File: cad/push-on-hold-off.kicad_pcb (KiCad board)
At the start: 2 copper layers, 22.9 x 12.7 mm, 17 parts, among them P1 CONN_01X04, P2 CONN_01X04, Q1 IRF7309IPBF, SW1 SW_PUSH_SMALL

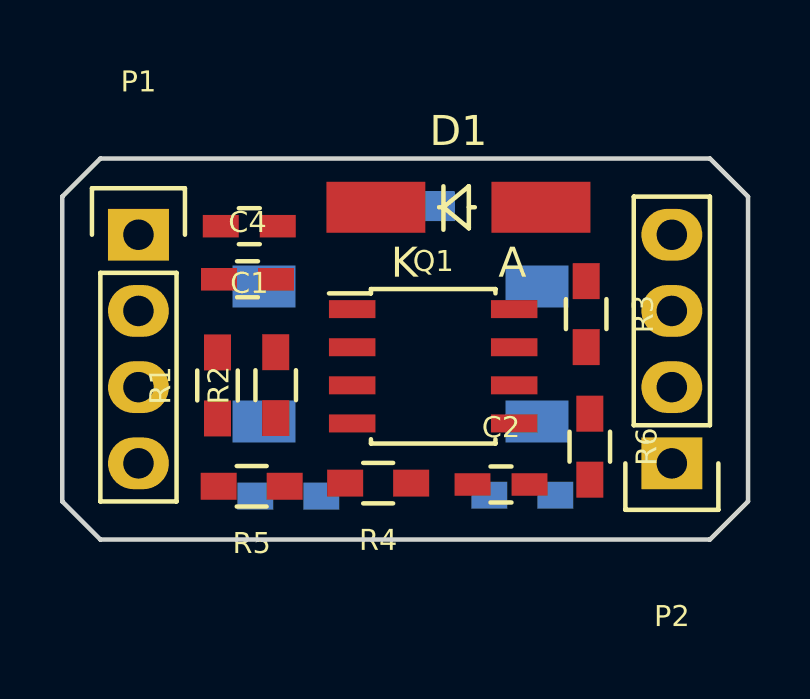
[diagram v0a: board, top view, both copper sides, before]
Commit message: Route the board
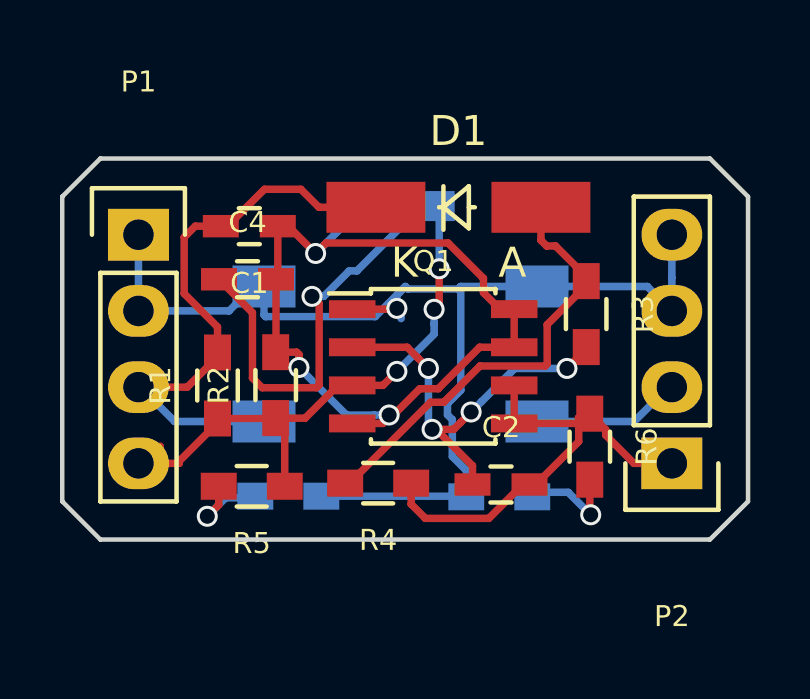
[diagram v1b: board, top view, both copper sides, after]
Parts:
- moved LED2 0.77 mm to (230.5, 111.6), turned to 0 degrees
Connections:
- C4 pad 1: /Vin -> Net-(C4-Pad1)
- JP1 pad 2: /Vin -> Net-(C4-Pad1)
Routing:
- net GND: track 0.00 -> 40.5 mm, vias 0 -> 1
- net Net-(C1-Pad1): track 0.00 -> 28.8 mm, vias 0 -> 3
- net /Button: track 0.00 -> 24.5 mm
- net /Vin: track 0.00 -> 19.7 mm, vias 0 -> 3
- net /Vout: track 0.00 -> 16.2 mm
- net Net-(D1-Pad2): track 0.00 -> 14.9 mm
- net Net-(C4-Pad1): track 0.00 -> 13.8 mm, vias 0 -> 1
- net Net-(C2-Pad1): track 0.00 -> 13.7 mm, vias 0 -> 4
- net Net-(LED2-Pad2): track 0.00 -> 3.77 mm, vias 0 -> 1
- net Net-(LED1-Pad2): track 0.00 -> 3.06 mm, vias 0 -> 1

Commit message: Sort out silkscreen and plot
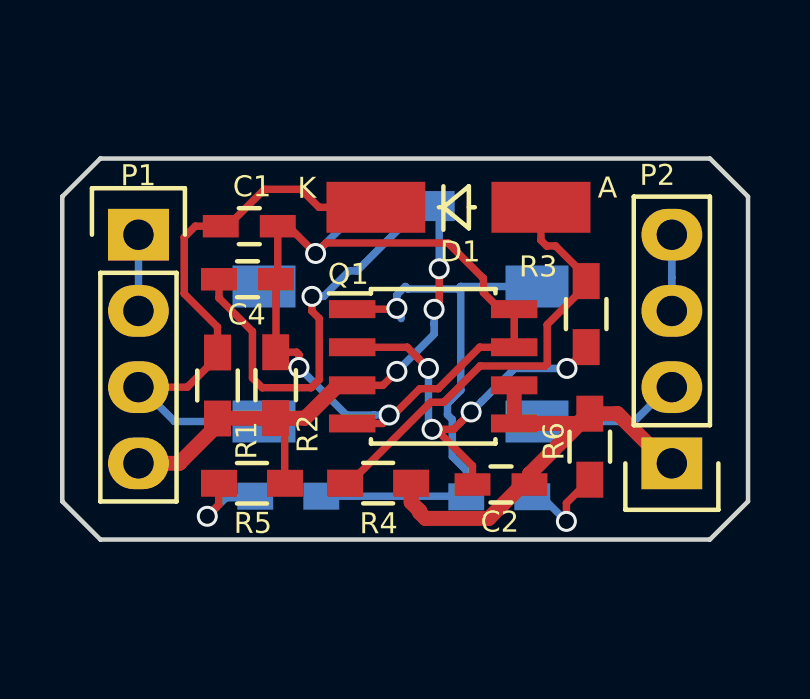
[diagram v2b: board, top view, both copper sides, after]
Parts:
- moved R5 0.10 mm to (222.2, 111.2)
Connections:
- C4 pad 1: Net-(C4-Pad1) -> /Vin
- JP1 pad 2: Net-(C4-Pad1) -> /Vin
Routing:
- net /Vin: track 19.7 -> 36.3 mm, vias 3 -> 4
- net GND: track 40.5 -> 25.2 mm
- net Net-(C4-Pad1): track 13.8 -> 0.00 mm, vias 1 -> 0
- net /Vout: track 16.2 -> 17.1 mm
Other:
- rule trace_min: 0.2 -> 0.1
